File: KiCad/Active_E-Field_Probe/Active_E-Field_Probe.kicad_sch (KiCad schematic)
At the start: 16 parts

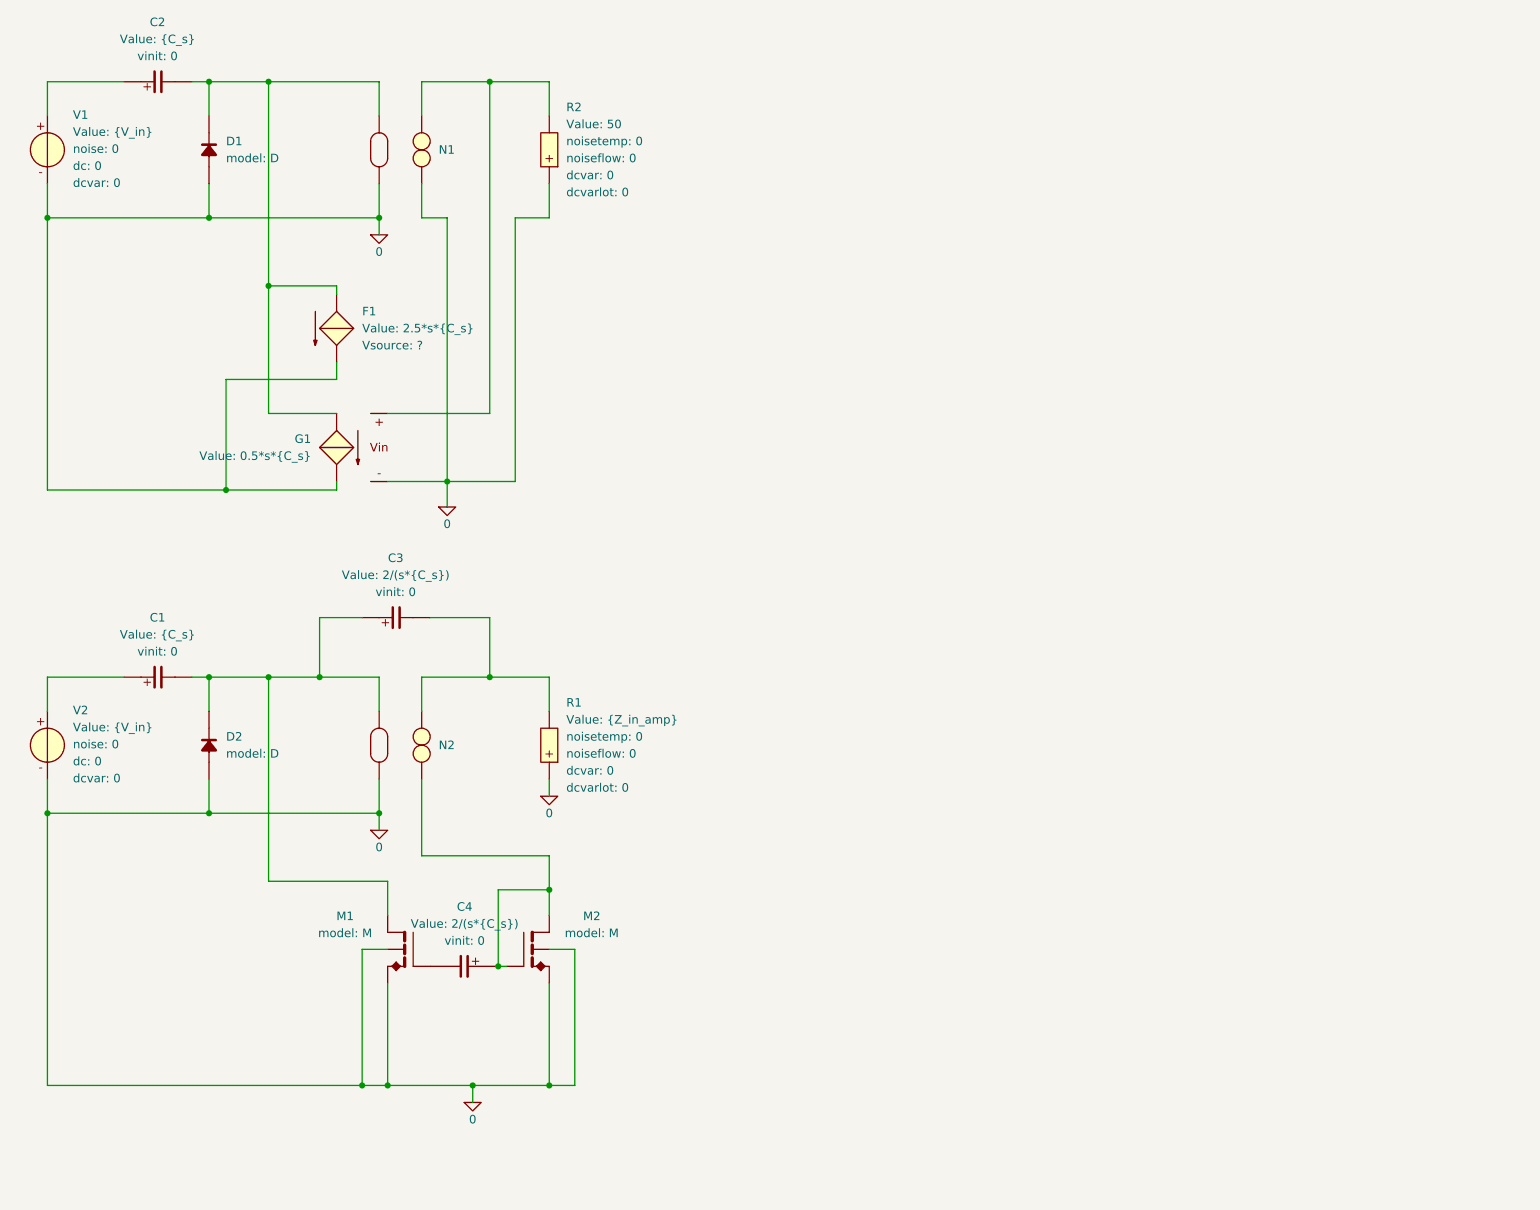
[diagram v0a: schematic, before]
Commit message: meeting 18-09
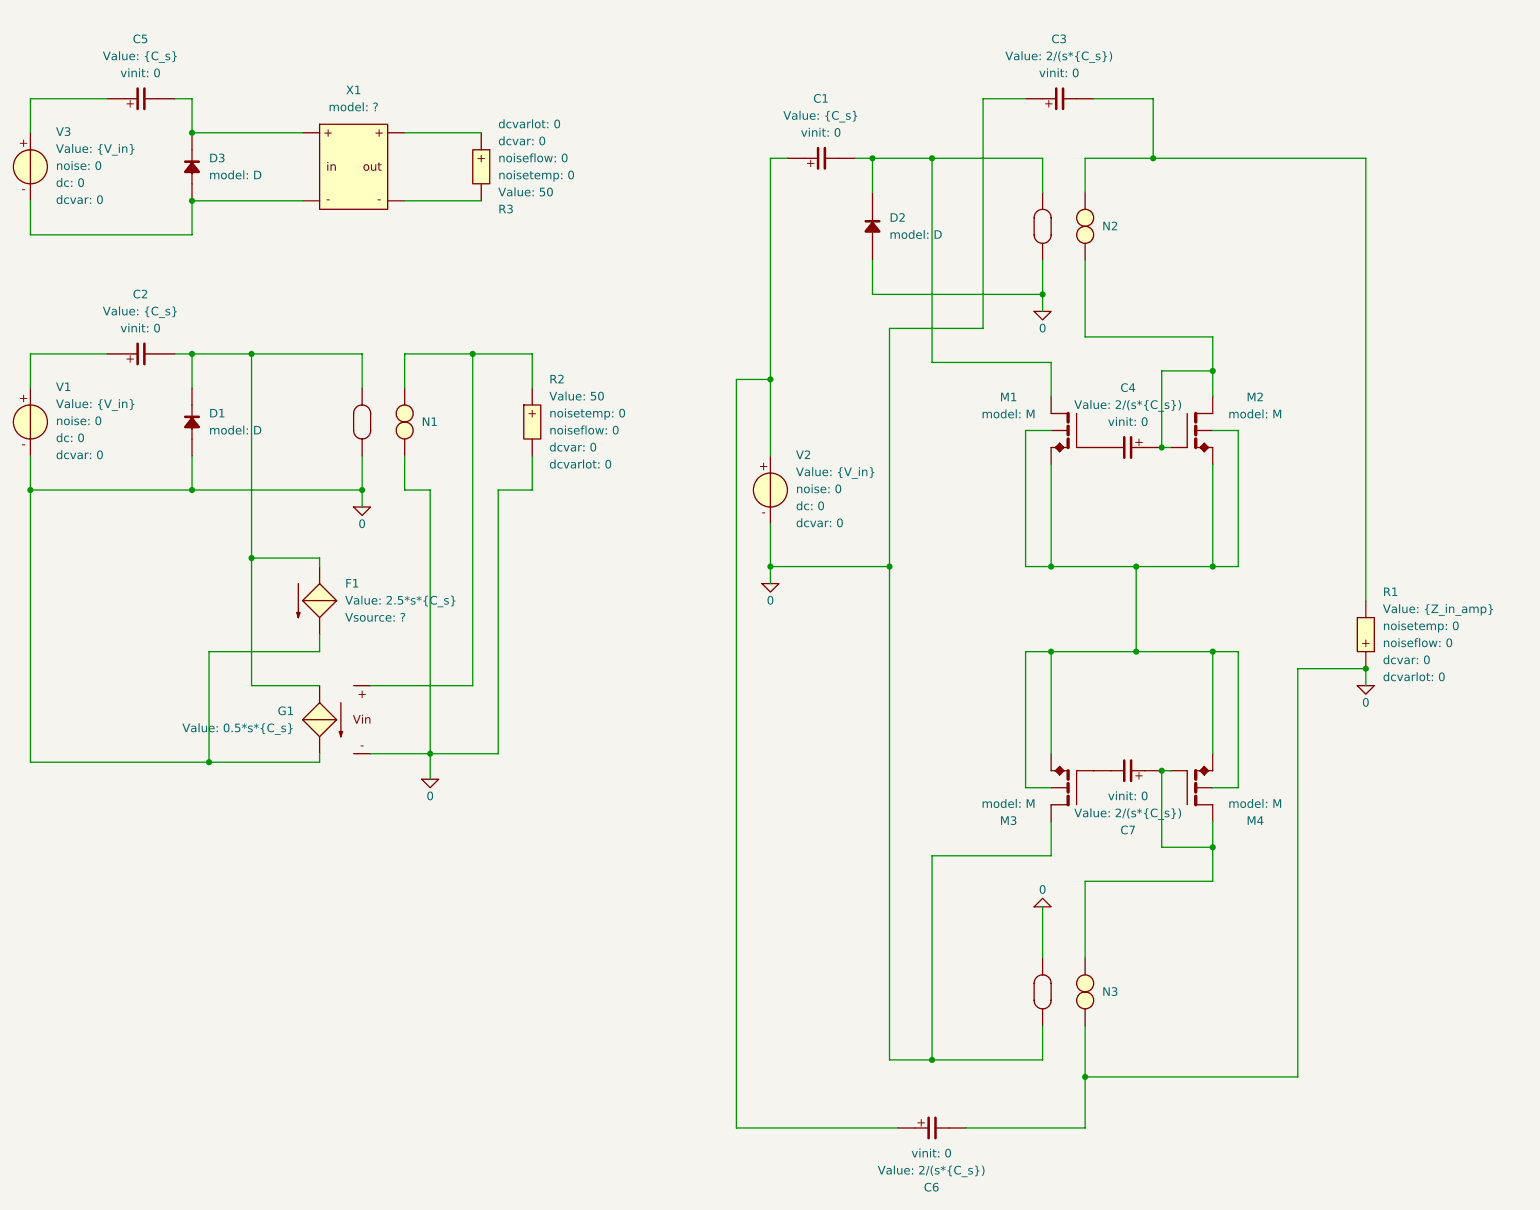
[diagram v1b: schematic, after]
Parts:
- added C5: {C_s}, symbol SLiCAP:C
- added C6, C7: 2/(s*{C_s}), symbol SLiCAP:C
- added D3: ~, symbol SLiCAP:D
- added M3, M4: ~, symbol SLiCAP:M
- added N3: ~, symbol SLiCAP:N
- added R3: 50, symbol SLiCAP:R
- added V3: {V_in}, symbol SLiCAP:V
- added X1: ~, symbol SLiCAP:Xio4
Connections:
- net 0: now also C3.1, R2.2, C6.2, M3.1 (D), N3.1 (outP), N3.3 (inp), N3.4 (inN); no longer M1.3 (S), M1.4 (B), M2.3 (S), M2.4 (B), R2.1
- net at C1.2, D2.2, M1.1 (D)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: no longer C3.1
- net at G1.3 (inp), N1.1 (outP): now also R2.1; no longer R2.2
- net at C1.1, V2.1 (p): now also C6.1
- new net: C7.1, M4.1 (D), M4.2 (G), N3.2 (outN)
- new net: C5.1, V3.1 (p)
- new net: C5.2, D3.2, X1.1 (inP)
- new net: C7.2, M3.2 (G)
- new net: D3.1, V3.2 (n), X1.2 (inN)
- new net: R3.1, X1.3 (outP)
- new net: R3.2, X1.4 (outN)
- new net: M1.3 (S), M1.4 (B), M2.3 (S), M2.4 (B), M3.3 (S), M3.4 (B), M4.3 (S), M4.4 (B)
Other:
- moved on the sheet: C1, C2, C3, C4, D1, D2, F1, G1, M1, M2, N1, N2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
